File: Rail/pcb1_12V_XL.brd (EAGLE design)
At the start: 96.3 x 101.8 mm, 116 parts, among them J1 638207222006, J10 638207222006, J11 638207222006, J12 638207222006, J2 638207222006, J4 61302211821, J8 61302211821, U1 ESP32-S3-DEVKITC-1-N8R2, U4 TLE9250VSJ, X2 B4P-VH

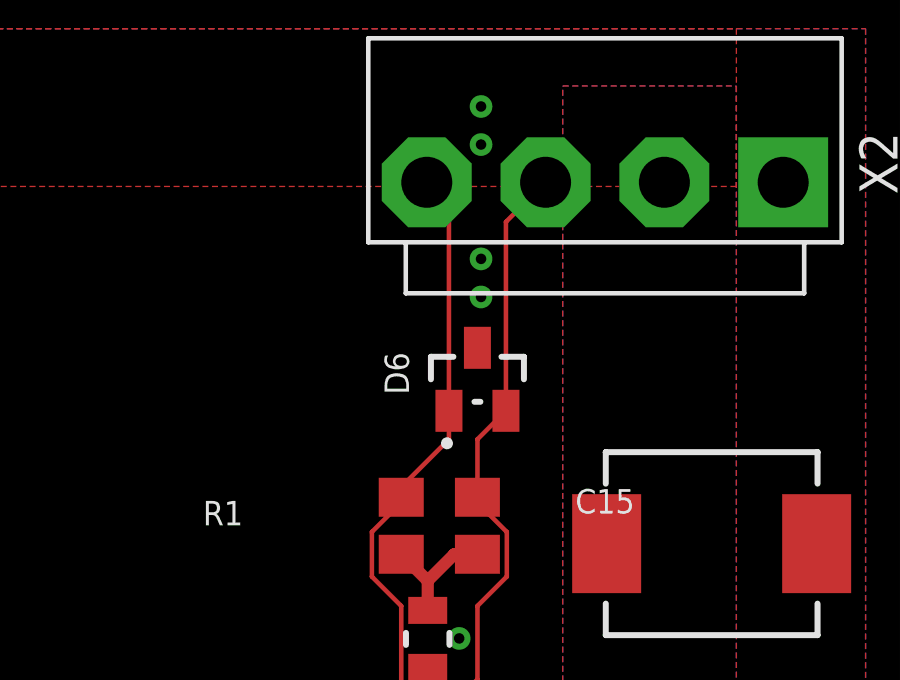
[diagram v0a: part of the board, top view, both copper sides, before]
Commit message: cleanup
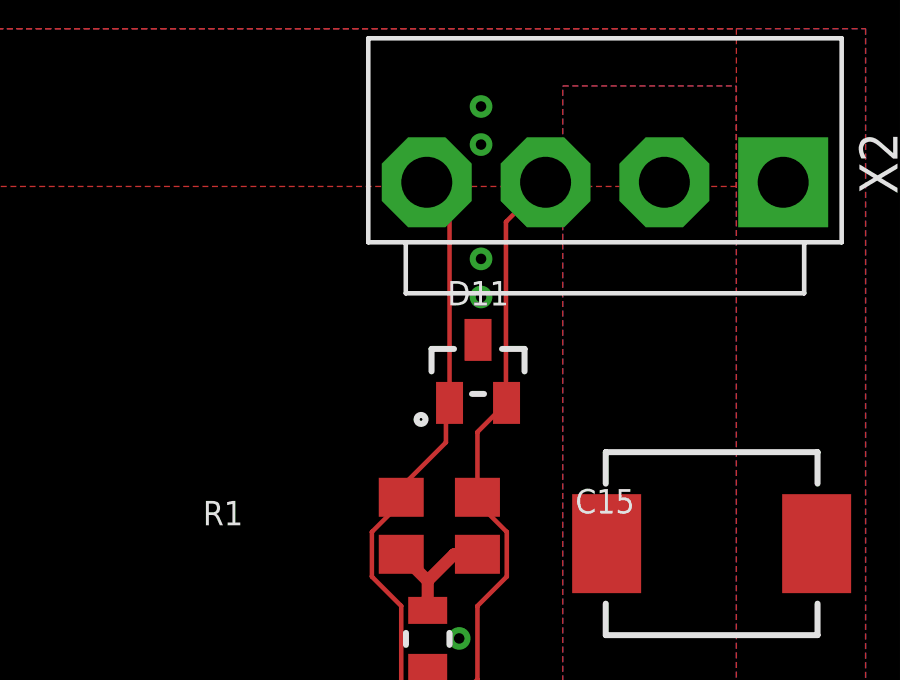
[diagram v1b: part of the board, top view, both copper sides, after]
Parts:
- removed D6: 26.2V / 35pF, fliegl-wuerth:WE-TVS_SOT23-3L
- added D11: 24Vdc, Wurth_EMC Components_WE-TVS:WE-TVS_SOT23-3L
- J4, J8: device Eagle_WR-PHD (rev22a):61302211821 -> Wurth_Connectors_WR-PHD:61302211821
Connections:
- net CAN_N: now also D11.1; no longer D6.1
- net CAN_P: now also D11.2; no longer D6.2
- net ECU_GND: now also D11.3; no longer D6.3
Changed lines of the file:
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@@
 <attribute name="VR" value="50V(DC)" x="82.9912" y="119.4" size="1.778" layer="27" rot="R270" display="off"/>
-</element>
-<element name="D6" library="fliegl-wuerth" package="WE-TVS_SOT23-3L" value="26.2V / 35pF" x="80.8388" y="87.4128" smashed="yes" rot="R90">
-<attribute name="ARTIKEL_NR" value="531887" x="73.2188" y="44.2328" size="1.778" layer="27" rot="R90" display="off"/>
-<attribute name="KOMPONENTENNUMMER" value="617684" x="73.2188" y="44.2328" size="1.778" layer="27" rot="R90" display="off"/>
-<attribute name="NAME" x="78.5568" y="87.6078" size="0.8128" layer="25" rot="R90" align="bottom-center"/>
-<attribute name="VALUE" x="83.4908" y="85.8078" size="0.6096" layer="27" rot="R90"/>
-<attribute name="WE-NUMBER" value="824098024" x="73.2188" y="44.2328" size="1.778" layer="27" rot="R90" display="off"/>
 </element>
 <element name="C17" library="Wurth_Capacitors_WCAP-CSGP" library_urn="urn:adsk.eagle:library:18488985" package="WCAP-CSGP_0805_H0.8_R" package3d_urn="urn:adsk.eagle:package:18489119/2" value="100nF" x="53.34" y="64.79" smashed="yes">
@@
 <attribute name="VALUE" x="-0.36" y="71.37" size="1.27" layer="27" rot="R270" align="top-left"/>
 </element>
-<element name="J4" library="Eagle_WR-PHD (rev22a)" package="61302211821" package3d_urn="urn:adsk.eagle:package:14805555/2" value=" 61302211821 " x="45.72" y="125.75" smashed="yes">
+<element name="J4" library="Wurth_Connectors_WR-PHD" library_urn="urn:adsk.eagle:library:14804658" package="61302211821" package3d_urn="urn:adsk.eagle:package:14805555/2" value=" 61302211821 " x="45.72" y="125.75" smashed="yes">
 <attribute name="DATASHEET-URL" value="https://www.we-online.com/redexpert/spec/61302211821?ae" x="15.24" y="195.6" size="1.778" layer="27" display="off"/>
 <attribute name="GENDER" value="Socket Header" x="15.24" y="195.6" size="1.778" layer="27" display="off"/>
@@
 <attribute name="VALUE" x="16.7224" y="124.5558" size="0.8128" layer="27" align="bottom-right"/>
 </element>
-<element name="J8" library="Eagle_WR-PHD (rev22a)" package="61302211821" package3d_urn="urn:adsk.eagle:package:14805555/2" value=" 61302211821 " x="45.72" y="120.67" smashed="yes">
+<element name="J8" library="Wurth_Connectors_WR-PHD" library_urn="urn:adsk.eagle:library:14804658" package="61302211821" package3d_urn="urn:adsk.eagle:package:14805555/2" value=" 61302211821 " x="45.72" y="120.67" smashed="yes">
 <attribute name="DATASHEET-URL" value="https://www.we-online.com/redexpert/spec/61302211821?ae" x="12.7" y="190.52" size="1.778" layer="27" display="off"/>
 <attribute name="GENDER" value="Socket Header" x="12.7" y="190.52" size="1.778" layer="27" display="off"/>
@@
 <attribute name="VBR" value="4.5V" x="38.1" y="60.96" size="1.778" layer="27" rot="R90" display="off"/>
 </element>
+<element name="D11" library="Wurth_EMC Components_WE-TVS" library_urn="urn:adsk.eagle:library:14282971" package="WE-TVS_SOT23-3L" package3d_urn="urn:adsk.eagle:package:12152380/4" value="24Vdc" x="80.858915625" y="87.675475" smashed="yes">
+<attribute name="C-CH" value="38pF" x="80.858915625" y="87.675475" size="1.778" layer="27" display="off"/>
+<attribute name="CHANNELS" value=" 2 " x="80.858915625" y="87.675475" size="1.778" layer="27" display="off"/>
+<attribute name="DATASHEET-URL" value="https://www.we-online.com/catalog/datasheet/824094024.pdf" x="80.858915625" y="87.675475" size="1.778" layer="27" display="off"/>
+<attribute name="IPEAK" value="6A" x="80.858915625" y="87.675475" size="1.778" layer="27" display="off"/>
+<attribute name="MOUNT" value="SMT" x="80.858915625" y="87.675475" size="1.778" layer="27" display="off"/>
+<attribute name="NAME" x="80.858915625" y="89.875475" size="0.8128" layer="25" align="bottom-center"/>
+<attribute name="PART-NUMBER" value=" 824094024 " x="80.858915625" y="87.675475" size="1.778" layer="27" display="off"/>
+<attribute name="VALUE" x="80.858915625" y="84.675475" size="0.8128" layer="27" align="bottom-center"/>
+<attribute name="VBR" value="26.2V" x="80.858915625" y="87.675475" size="1.778" layer="27" display="off"/>
+</element>
 </elements>
 <signals>
@@
 <signal name="CAN_P">
 <contactref element="U4" pad="7"/>
-<contactref element="D6" pad="2"/>
 <contactref element="R1" pad="2"/>
 <contactref element="X2" pad="3"/>
 <wire x1="83.11" y1="93.98" x2="81.7888" y2="92.6588" width="0.1524" layer="1"/>
-<wire x1="81.7888" y1="92.6588" x2="81.7888" y2="86.3628" width="0.1524" layer="1"/>
 <wire x1="54.61" y1="59.69" x2="62.23" y2="59.69" width="0.1524" layer="1"/>
 <wire x1="62.23" y1="59.69" x2="78.58025" y2="76.04025" width="0.1524" layer="1"/>
@@
 <wire x1="53.4924" y1="58.5724" x2="54.61" y2="59.69" width="0.1524" layer="1"/>
 <wire x1="53.4924" y1="57.8324" x2="53.4924" y2="58.5724" width="0.1524" layer="1"/>
-<wire x1="81.7888" y1="86.3628" x2="80.8388" y2="85.4128" width="0.1524" layer="1"/>
-<wire x1="80.8388" y1="85.4128" x2="80.8388" y2="83.48" width="0.1524" layer="1"/>
 <wire x1="80.8388" y1="83.48" x2="80.8388" y2="83.3032875" width="0.1524" layer="1"/>
 <wire x1="80.8388" y1="83.3032875" x2="81.8174" y2="82.3246875" width="0.1524" layer="1"/>
@@
 <wire x1="80.8388" y1="77.4093125" x2="79.4697375" y2="76.04025" width="0.1524" layer="1"/>
 <wire x1="79.4697375" y1="76.04025" x2="78.58025" y2="76.04025" width="0.1524" layer="1"/>
+<contactref element="D11" pad="2"/>
+<wire x1="80.8388" y1="85.655359375" x2="81.808915625" y2="86.625475" width="0.1524" layer="1"/>
+<wire x1="80.8388" y1="83.48" x2="80.8388" y2="85.655359375" width="0.1524" layer="1"/>
+<wire x1="81.7888" y1="92.6588" x2="81.7888" y2="86.645590625" width="0.1524" layer="1"/>
+<wire x1="81.7888" y1="86.645590625" x2="81.808915625" y2="86.625475" width="0.1524" layer="1"/>
 </signal>
 <signal name="CAN_N">
 <contactref element="U4" pad="6"/>
-<contactref element="D6" pad="1"/>
 <contactref element="R3" pad="2"/>
 <wire x1="78.2988" y1="83.48" x2="78.2988" y2="83.82" width="0.254" layer="1"/>
 <contactref element="X2" pad="4"/>
-<wire x1="79.15" y1="93.98" x2="79.8888" y2="93.2412" width="0.1524" layer="1"/>
-<wire x1="79.8888" y1="93.2412" x2="79.8888" y2="86.3628" width="0.1524" layer="1"/>
 <wire x1="62.1037375" y1="59.9948" x2="78.2988" y2="76.1898625" width="0.1524" layer="1"/>
 <wire x1="54.48374375" y1="59.9948" x2="62.1037375" y2="59.9948" width="0.1524" layer="1"/>
@@
 <wire x1="54.48374375" y1="59.9948" x2="54.394475" y2="59.90553125" width="0.1524" layer="1"/>
 <wire x1="54.394475" y1="59.90553125" x2="54.39446875" y2="59.90553125" width="0.1524" layer="1"/>
-<wire x1="79.8888" y1="86.3628" x2="79.8888" y2="85.41" width="0.1524" layer="1"/>
-<wire x1="79.8888" y1="85.41" x2="78.2988" y2="83.82" width="0.1524" layer="1"/>
+<wire x1="79.7894" y1="85.3106" x2="78.2988" y2="83.82" width="0.1524" layer="1"/>
 <wire x1="78.2988" y1="83.48" x2="78.2988" y2="83.3032875" width="0.1524" layer="1"/>
 <wire x1="78.2988" y1="83.3032875" x2="77.3202" y2="82.3246875" width="0.1524" layer="1"/>
@@
 <wire x1="77.3202" y1="80.8353125" x2="78.2988" y2="79.8567125" width="0.1524" layer="1"/>
 <wire x1="78.2988" y1="79.8567125" x2="78.2988" y2="76.1898625" width="0.1524" layer="1"/>
+<contactref element="D11" pad="1"/>
+<wire x1="79.908915625" y1="93.221084375" x2="79.908915625" y2="86.625475" width="0.1524" layer="1"/>
+<wire x1="79.15" y1="93.98" x2="79.908915625" y2="93.221084375" width="0.1524" layer="1"/>
+<wire x1="79.7894" y1="85.3106" x2="79.7894" y2="86.505959375" width="0.1524" layer="1"/>
+<wire x1="79.7894" y1="86.505959375" x2="79.908915625" y2="86.625475" width="0.1524" layer="1"/>
 </signal>
 <signal name="+3V3">
@@
 <contactref element="C10" pad="1"/>
 <contactref element="C15" pad="2"/>
-<contactref element="D6" pad="3"/>
 <contactref element="C17" pad="2"/>
 <contactref element="C19" pad="2"/>
@@
 <contactref element="J2" pad="A5"/>
 <contactref element="J2" pad="5"/>
+<contactref element="D11" pad="3"/>
 </signal>
 <signal name="IX00">
@@
 <mfgpreviewcolor name="substratecolor" color="0xFF786E46"/>
 </mfgpreviewcolors>
-<errors>
-</errors>
 </board>
 </drawing>
